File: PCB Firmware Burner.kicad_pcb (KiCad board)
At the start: 2 copper layers, 34.7 x 35.3 mm, 28 parts, among them J2 Conn_01x07_Male, Q1 BSS138, Q2 BSS138, T5V0b1 T5V0b1, T5V0b2 T5V0b2, T5V0c1 T5V0c1, T5V0c2 T5V0c2

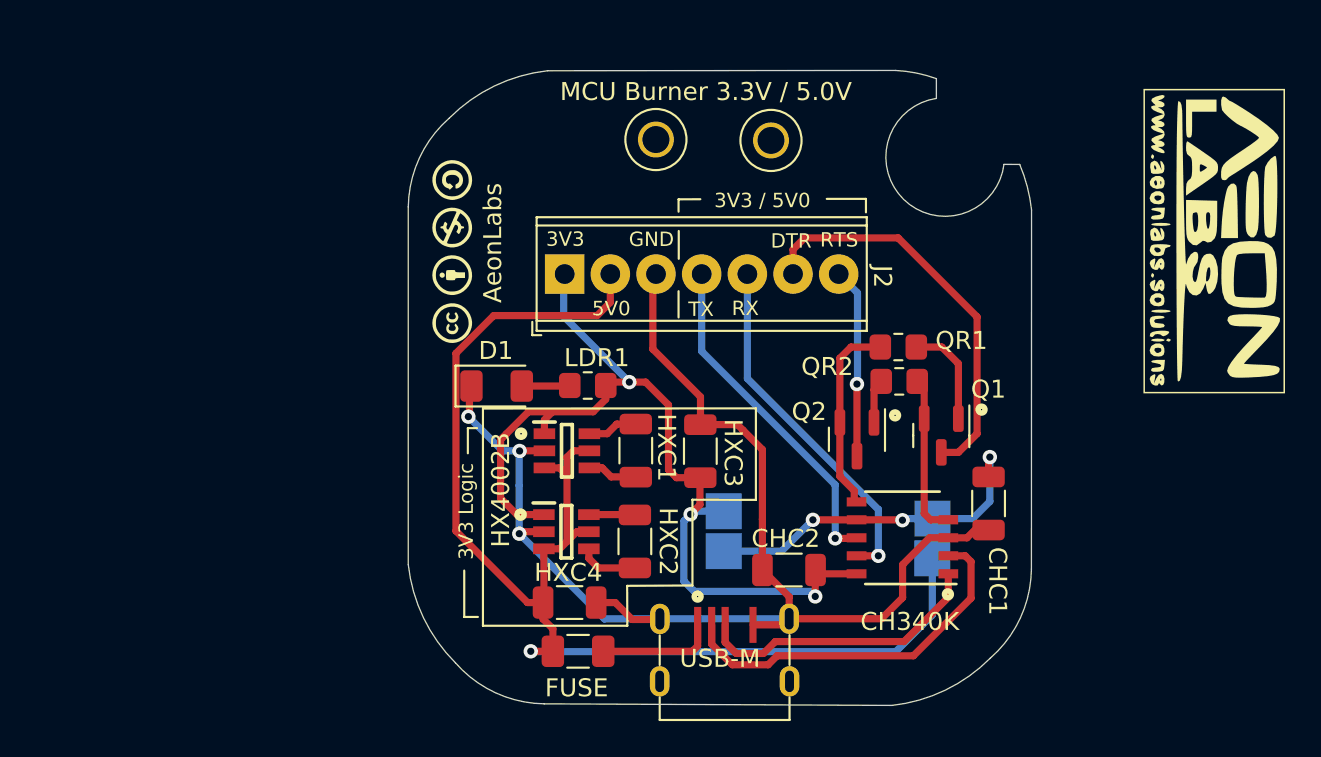
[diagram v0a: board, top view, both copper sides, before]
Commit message: rev 1.4
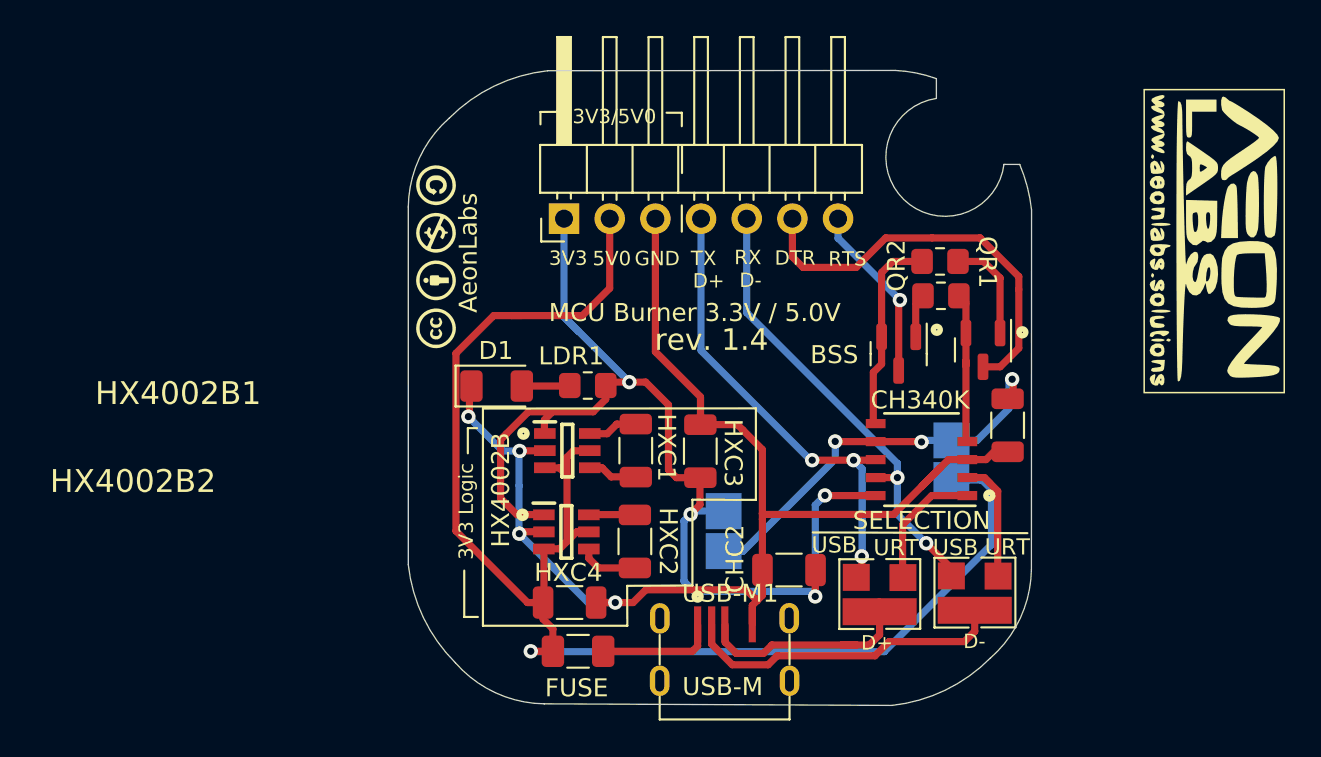
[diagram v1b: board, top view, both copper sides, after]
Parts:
- removed REF** (x2): TestPoint_Plated_Hole_D2.0mm, TestPoint:TestPoint_Plated_Hole_D2.0mm
- added TP3: TP_3Pole, TestPoint:TestPoint_Pad_1.5mm 3 points, F.Cu at (172.9, 100.9)
- added TP4: TP_3Pole, TestPoint:TestPoint_Pad_1.5mm 3 points, F.Cu at (178.2, 100.9)
- J2: footprint TerminalBlock_Phoenix:TerminalBlock_Phoenix_MPT-0,5-7-2.54_1x07_P2.54mm_Horizontal -> Connector_PinHeader_2.54mm:PinHeader_1x07_P2.54mm_Horizontal
- moved G*** 12.8 mm to (163.9, 91.2)
- moved QR1 5.30 mm to (176.5, 82.2)
- moved BSS 5.30 mm to (174.2, 87.3)
- moved Q1 5.30 mm to (178.9, 87.1)
- moved QR2 5.30 mm to (176.5, 84.1)
- moved CH340K1 4.48 mm to (175.5, 93.2)
- moved CHC1 4.48 mm to (180.2, 91.3)
- moved T5V0b1 4.48 mm to (177.1, 94.3)
- moved T5V0c1 4.48 mm to (177.1, 92.1)
- moved G*** 3.85 mm to (163.5, 85.1)
- moved J2 3.08 mm to (155.6, 79.8), turned to 90 degrees
- moved G*** 0.95 mm to (148.4, 81.9)
- renumbered Q2 to BSS
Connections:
- USB-M1 pad 2: Net-(CH340K1-Pad2) -> Net-(TP4-Pad1)
- USB-M1 pad 3: Net-(CH340K1-Pad1) -> Net-(TP3-Pad1)
- USB-M1 pad 6: /GND -> unconnected-(USB-M1-Pad6)
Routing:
- net Net-(TP4-Pad1): track 0.00 -> 19.1 mm
- net Net-(CH340K1-Pad2): track 20.9 -> 6.70 mm
- net Net-(TP3-Pad1): track 0.00 -> 13.5 mm
- net /HX3V3: track 52.1 -> 62.9 mm, vias 3 -> 4
- net /5V0: track 71.5 -> 81.9 mm
- net Net-(CH340K1-Pad1): track 16.2 -> 6.64 mm
- net /TX_OUT_3V3: track 19.2 -> 26.5 mm, vias 1 -> 3
- net /RX_OUT_3V3: track 20.1 -> 25.2 mm, vias 1 -> 2
- net Net-(CH340K1-Pad7): track 19.6 -> 22.6 mm
- net /GND: track 72.4 -> 71.4 mm, vias 3 -> 4
- net Net-(CH340K1-Pad4): track 9.00 -> 8.01 mm
- net Net-(Q2-Pad1): track 2.59 -> 1.82 mm
- net /RST_EN_RTS: track 10.6 -> 9.96 mm
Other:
- board text added: "3V0"
- board text added: "3V3/5V0"
- board text added: "Copyright 2022"
- board text added: "D+"
- board text added: "D-"
- board text added: "SELECTION"
- board text added: "URT"
- board text added: "USB"
- board text added: "rev. 1.4"
- board text removed: "3V3 / 5V0"
- board text removed: "Copyright 2022 rev. 1.3"
- board text removed: "EN 3V0"
- board text removed: "EN 5V0"
